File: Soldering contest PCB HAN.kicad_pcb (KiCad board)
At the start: 2 copper layers, 99 x 99 mm, 13 parts, among them J1 Screw_Terminal_01x02, Q1 2N3904, Q2 2N3904

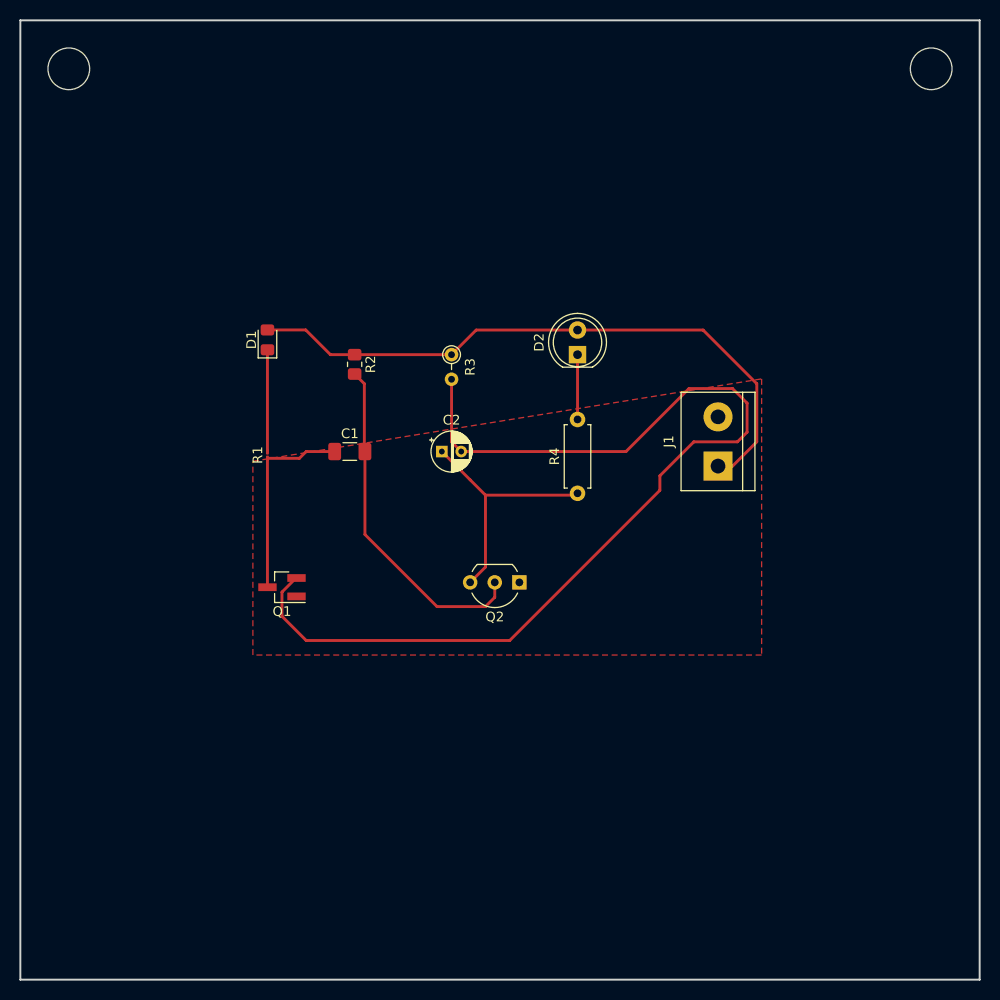
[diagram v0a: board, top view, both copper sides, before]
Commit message: started on silkscreen
added student and grade boxes
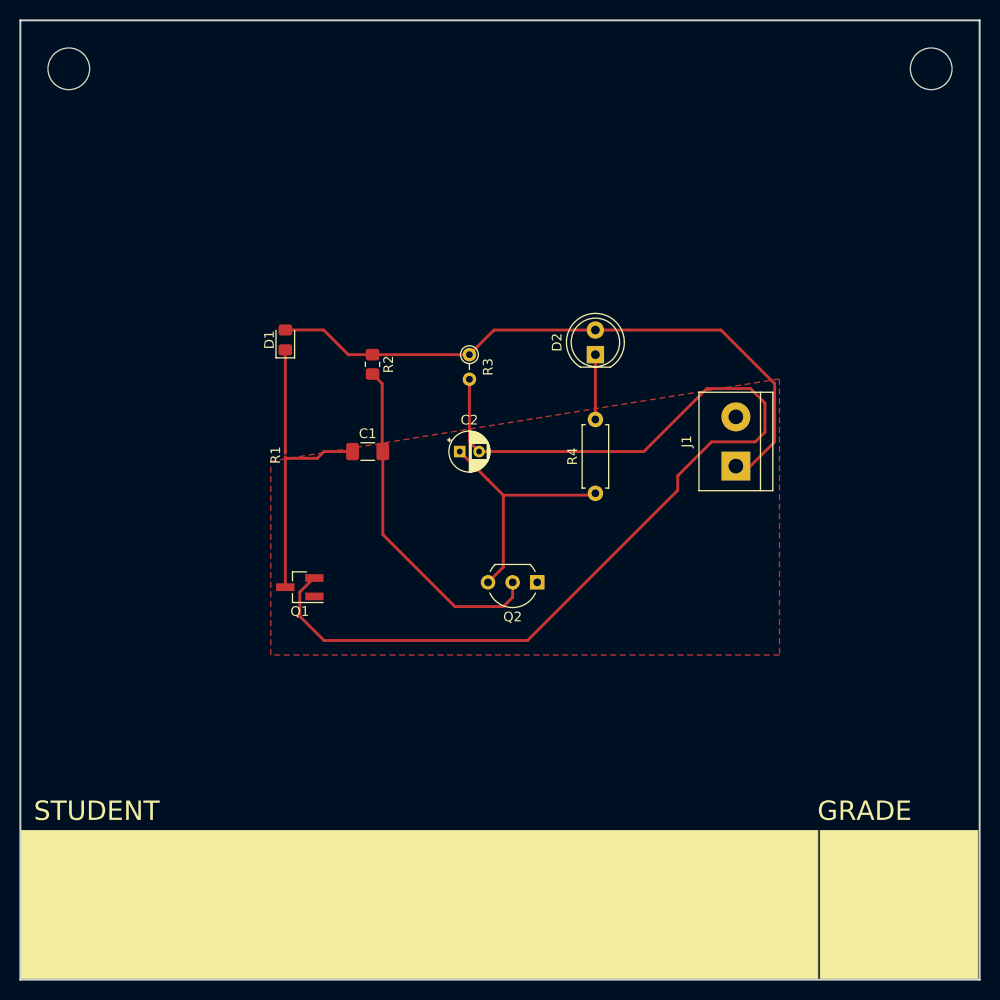
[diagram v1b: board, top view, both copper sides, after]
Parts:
- moved C1 1.84 mm to (147.3, 95.5)
- moved C2 1.84 mm to (156.8, 95.5)
- moved D1 1.84 mm to (138.8, 84.0)
- moved D2 1.84 mm to (170.8, 85.5)
- moved J1 1.84 mm to (185.3, 97.0)
- moved Q1 1.84 mm to (140.3, 109.5)
- moved Q2 1.84 mm to (164.8, 109.0)
- moved R1 1.84 mm to (138.8, 95.9)
- moved R2 1.84 mm to (147.8, 86.5)
- moved R3 1.84 mm to (157.8, 85.5)
- moved R4 1.84 mm to (170.8, 99.8)
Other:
- board text added: "GRADE"
- board text added: "STUDENT"
